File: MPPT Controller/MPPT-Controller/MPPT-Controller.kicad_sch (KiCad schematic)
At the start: 50 parts, among them J1 Conn_01x02_Pin, J2 Conn_01x02_Pin, J3 Conn_01x02_Pin, J4 Conn_01x02_Pin, J6 Conn_01x02_Pin, Q1 IRL540N, SW1 SW_SPDT, U1 ADS1115IDGS, U4 LM1117DT-3.3, U5 LM2596S-ADJ, U6 TC4422, U7 ADS1115IDGS

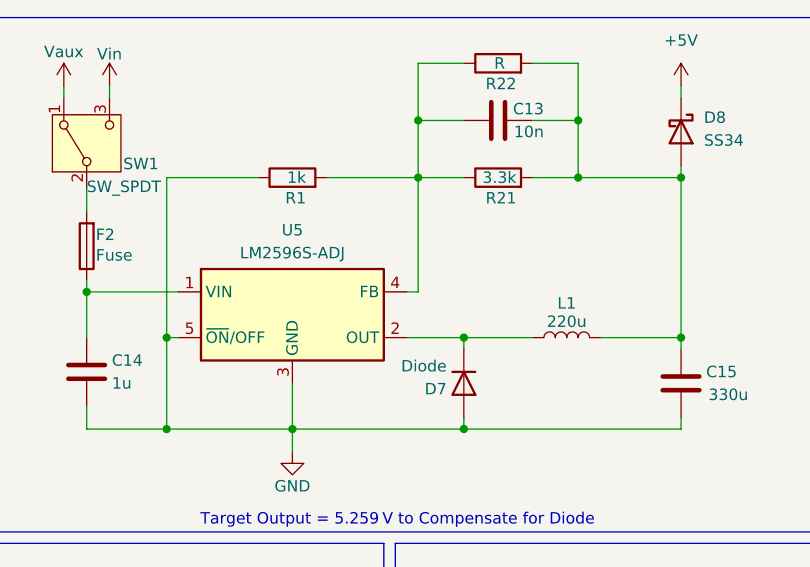
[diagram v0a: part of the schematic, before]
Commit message: Compact
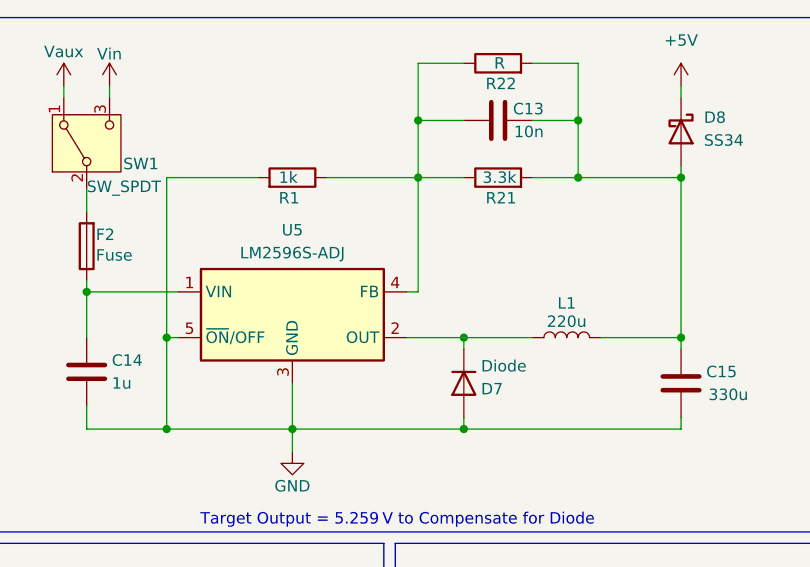
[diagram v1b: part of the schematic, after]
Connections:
- net GND: now also R1.2; no longer R1.1
- net at C13.1, R21.1, R22.1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: now also R1.1; no longer R1.2
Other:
- moved on the sheet: D7, R1
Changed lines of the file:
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@@
 	(symbol
 		(lib_id "Device:R")
-		(at 160.02 31.75 90)
+		(at 160.02 31.75 270)
+		(mirror x)
 		(unit 1)
 		(exclude_from_sim no)
@@
 		(dnp no)
 		(property "Reference" "R1"
-			(at 161.544 34.036 90)
+			(at 158.496 34.036 90)
 			(effects
 				(font
@@
 		)
 		(property "Value" "1k"
-			(at 161.544 31.75 90)
+			(at 158.496 31.75 90)
 			(effects
 				(font
@@
 	(symbol
 		(lib_id "ScottoKeebs:Placeholder_Diode")
-		(at 179.07 54.61 270)
+		(at 179.07 54.61 90)
+		(mirror x)
 		(unit 1)
 		(exclude_from_sim no)
@@
 		(dnp no)
 		(property "Reference" "D7"
-			(at 177.165 55.245 90)
+			(at 180.975 55.245 90)
 			(effects
 				(font
@@
 		)
 		(property "Value" "Diode"
-			(at 177.165 52.705 90)
-			(effects
-				(font
+			(at 180.975 52.705 90)
+			(effects
+				(font
